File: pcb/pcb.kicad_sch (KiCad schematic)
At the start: 128 parts, among them U1 ProMicro

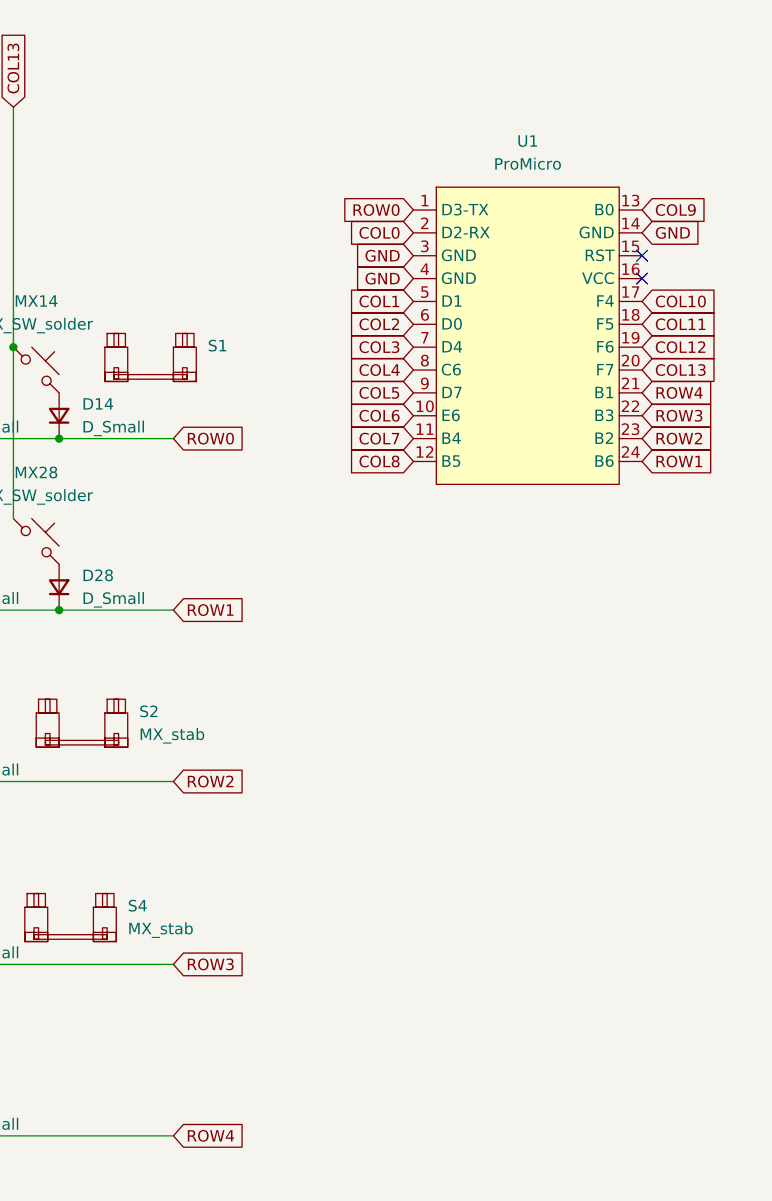
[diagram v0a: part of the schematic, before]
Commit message: sleep
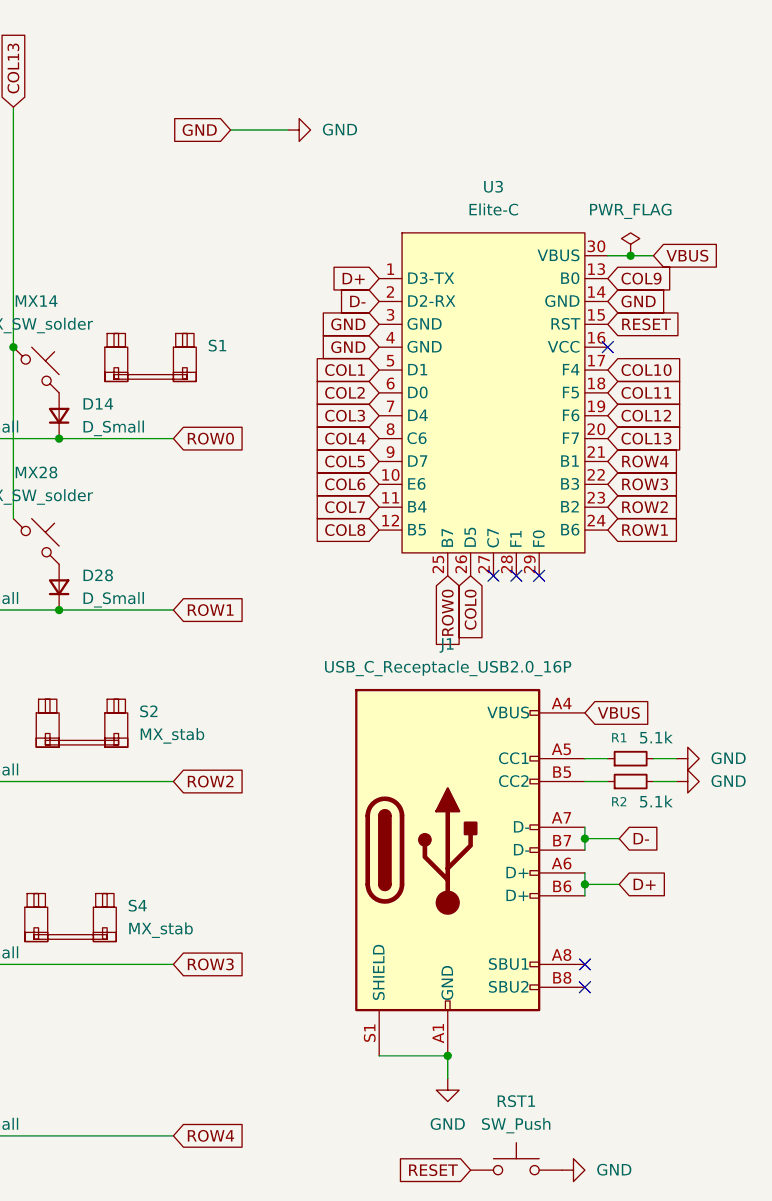
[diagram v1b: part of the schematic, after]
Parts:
- removed U1: ProMicro, PCM_marbastlib-xp-promicroish:ProMicro_USBup, symbol PCM_marbastlib-promicroish:Arduino_ProMicro
- added J1: USB_C_Receptacle_USB2.0_16P, Connector_USB:USB_C_Receptacle_HRO_TYPE-C-31-M-12, symbol Connector:USB_C_Receptacle_USB2.0_16P
- added R1, R2: 5.1k, Resistor_SMD:R_0402_1005Metric, symbol Device:R_Small
- added RST1: SW_Push, Button_Switch_SMD:SW_SPST_TL3305B, symbol Switch:SW_Push
- added U3: Elite-C, PCM_marbastlib-xp-promicroish:Elite-C_ACH, symbol PCM_marbastlib-promicroish:Elite-C
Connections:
- net COL0: now also U3.26 (D5)
- net COL1: now also U3.5 (D1)
- net COL10: now also U3.17 (F4)
- net COL11: now also U3.18 (F5)
- net COL12: now also U3.19 (F6)
- net COL13: now also U3.20 (F7)
- net COL2: now also U3.6 (D0)
- net COL3: now also U3.7 (D4)
- net COL4: now also U3.8 (C6)
- net COL5: now also U3.9 (D7)
- net COL6: now also U3.10 (E6)
- net COL7: now also U3.11 (B4)
- net COL8: now also U3.12 (B5)
- net COL9: now also U3.13 (B0)
- net GND: now also J1.A1 (GND), J1.A12 (GND), J1.B1 (GND), J1.B12 (GND), J1.S1 (SHIELD), R1.2, R2.2, RST1.2, U3.14 (GND), U3.3 (GND), U3.4 (GND)
- net ROW0: now also U3.25 (B7)
- net ROW1: now also U3.24 (B6)
- net ROW2: now also U3.23 (B2)
- net ROW3: now also U3.22 (B3)
- net ROW4: now also U3.21 (B1)
- new net: J1.A5 (CC1), R1.1
- new net: J1.B5 (CC2), R2.1
- new net D+: J1.A6 (D+), J1.B6 (D+), U3.1 (D3-TX)
- new net D-: J1.A7 (D-), J1.B7 (D-), U3.2 (D2-RX)
- new net RESET: RST1.1, U3.15 (RST)
- new net VBUS: J1.A4 (VBUS), J1.A9 (VBUS), J1.B4 (VBUS), J1.B9 (VBUS), U3.30 (VBUS)
- no-connect marks 2 -> 6
